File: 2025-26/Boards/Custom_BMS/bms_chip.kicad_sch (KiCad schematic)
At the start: 53 parts, among them CN1 C4201WR-F-2X8P_C5355564, CN2 0530470210, CN3 0530470210, CN7 530470610, Q1 ZXTN4004KTC, U1 BQ79616PAPRQ1

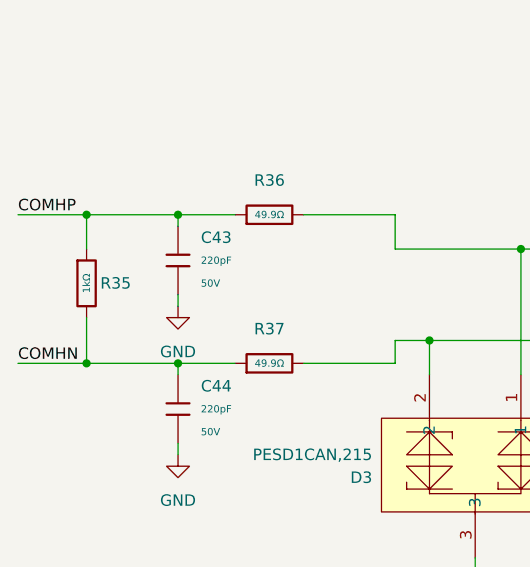
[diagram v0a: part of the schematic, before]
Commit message: more gnding changes
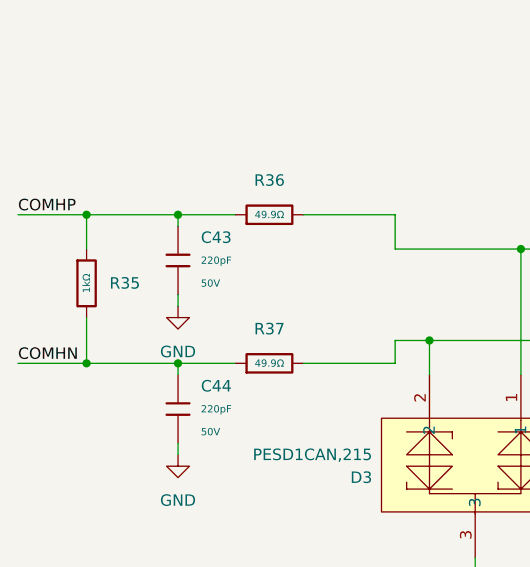
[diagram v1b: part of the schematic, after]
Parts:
- removed R35, R38: 1kΩ, PCM_JLCPCB:R_0603, symbol PCM_JLCPCB-Resistors:0603,1kΩ
- added R35, R38: 1kΩ, PCM_JLCPCB:R_0402, symbol PCM_JLCPCB-Resistors:0402,1kΩ
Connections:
- net COMHN: now also R35.2
- net COMHP: now also R35.1
- net COMLN: now also R38.2
- net COMLP: now also R38.1
